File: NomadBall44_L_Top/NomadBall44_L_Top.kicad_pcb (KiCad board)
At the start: 2 copper layers, 149 x 96.5 mm, 58 parts, among them SW1 SW_Push, SW10 SW_Push, SW11 SW_Push, SW12 SW_Push, SW13 SW_Push, SW14 SW_Push, SW15 SW_Push, SW16 SW_Push, SW17 SW_Push, SW18 SW_Push, SW19 SW_Push, SW2 SW_Push, SW20 SW_Push, SW21 SW_Push, SW22 SW_Push, SW23 SW_Push, SW24 SW_SPDT, SW3 SW_Push, SW4 SW_Push, SW5 SW_Push, SW6 SW_Push, SW7 SW_Push, SW8 SW_Push, SW9 SW_Push, U1 XIAO-nRF52840-Plus-SMD

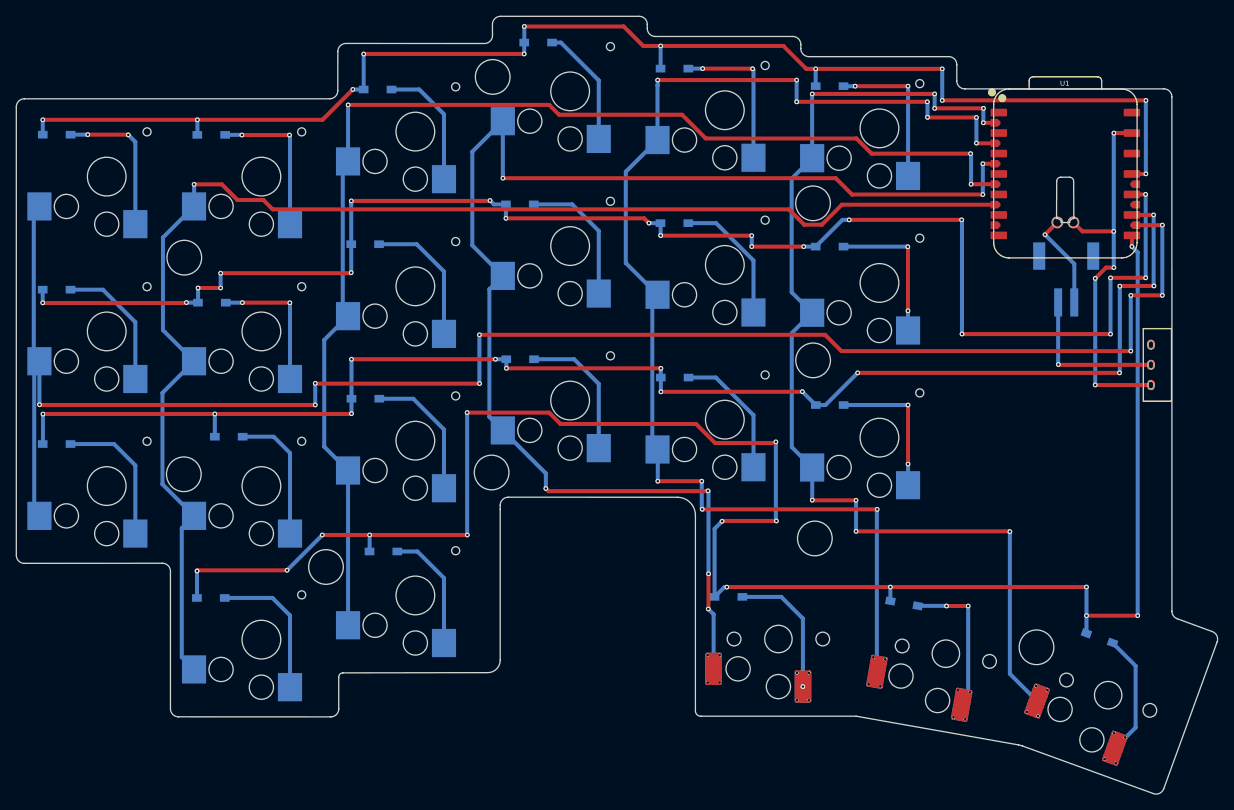
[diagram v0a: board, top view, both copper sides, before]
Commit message: トッププレート完成
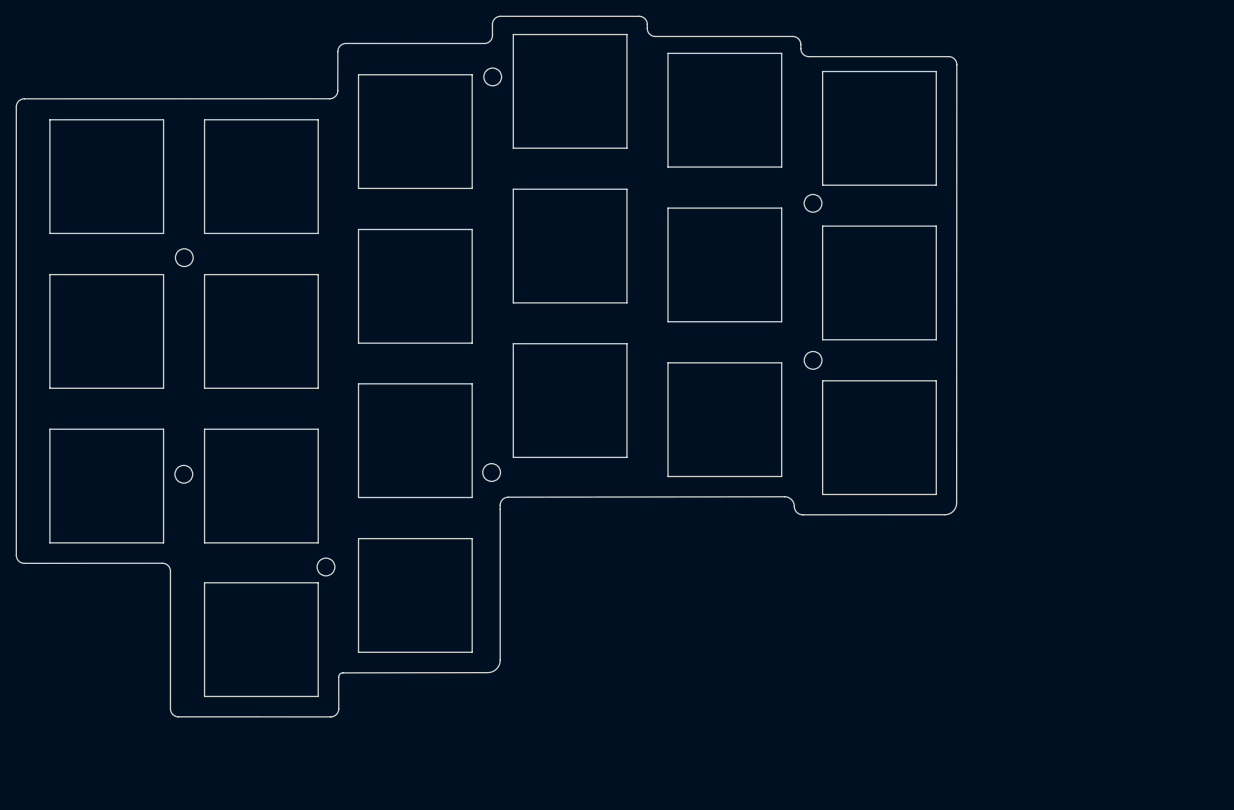
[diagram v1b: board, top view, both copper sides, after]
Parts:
- removed BT1: Battery_Cell, NomadBall44:JST_S2B-PH-SM4-TB
- removed D1, D10, D11, D12, D13, D14, D15, D16, D17, D18, D19, D2, D20, D21, D22, D23, D3, D4, D5, D6, D7, D8, D9: D, NomadBall44:Diode_SMD
- removed the REF** at (230.9, 119.9)
- removed the REF** at (258.4, 133.4)
- removed SW19, SW20, SW21: SW_Push, NomadBall44:Kailh_Choc_V1_Hotswap_thin_via
- removed SW24: SW_SPDT, NomadBall44:TGSW_MSK-12D19
- removed U1: XIAO-nRF52840-Plus-SMD, NomadBall44:XIAO-nRF52840-Plus-ver2
- REF** (x7): value MountingHole_4.3mm_M4 -> Val**; footprint MountingHole:MountingHole_4.3mm_M4 -> NomadBall44:m2_Screw_Hole
- SW1, SW10, SW11, SW12, SW13, SW14, SW15, SW16, SW17, SW18, SW2, SW22, SW23, SW3, SW4, SW5, SW6, SW7, SW8, SW9: footprint NomadBall44:Choc_v2_Hotswap_1u -> NomadBall44:SW_Hole_1u
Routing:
- net Row3: track 230.2 -> 0.00 mm, vias 15 -> 0
- net Col5: track 212.8 -> 0.00 mm, vias 9 -> 0
- net Row1: track 190.7 -> 0.00 mm, vias 21 -> 0
- net Row2: track 179.8 -> 0.00 mm, vias 14 -> 0
- net Row0: track 171.8 -> 0.00 mm, vias 12 -> 0
- net Col4: track 170.4 -> 0.00 mm, vias 1 -> 0
- net Col2: track 167.8 -> 0.00 mm, vias 7 -> 0
- net Col1: track 154.1 -> 0.00 mm, vias 11 -> 0
- net Col3: track 154.1 -> 0.00 mm, vias 3 -> 0
- net Col0: track 131.7 -> 0.00 mm, vias 9 -> 0
- net GND: track 47.4 -> 0.00 mm, vias 5 -> 0
- net Net-(BT1--): track 19.2 -> 0.00 mm, vias 1 -> 0
- net Net-(D1-A): track 19.1 -> 0.00 mm, vias 2 -> 0
- net Net-(D5-A): track 19.1 -> 0.00 mm, vias 2 -> 0
- net Net-(D2-A): track 19.1 -> 0.00 mm, vias 2 -> 0
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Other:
- board size 149 x 96.5 mm -> 116.7 x 86.9 mm
